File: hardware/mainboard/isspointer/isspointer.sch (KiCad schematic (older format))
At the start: 83 parts, among them J1 USB_B_Micro, J2 Motor 1, J3 Motor 2, Q1 SS8050-G, Q2 SS8050-G, Q3 DMN67D8L, Q4 DMN67D8L, SW1 SW_Push, SW2 SW_Push, U1 AMS1117-3.3, U2 CP2102N-A01-GQFN28, U3 esp32-WROOM-32D, U4 DRV8834_HTSSOP, U5 DRV8834_HTSSOP, U6 LSM303DLHC, U7 EE-SX3350, U8 EE-SX3350

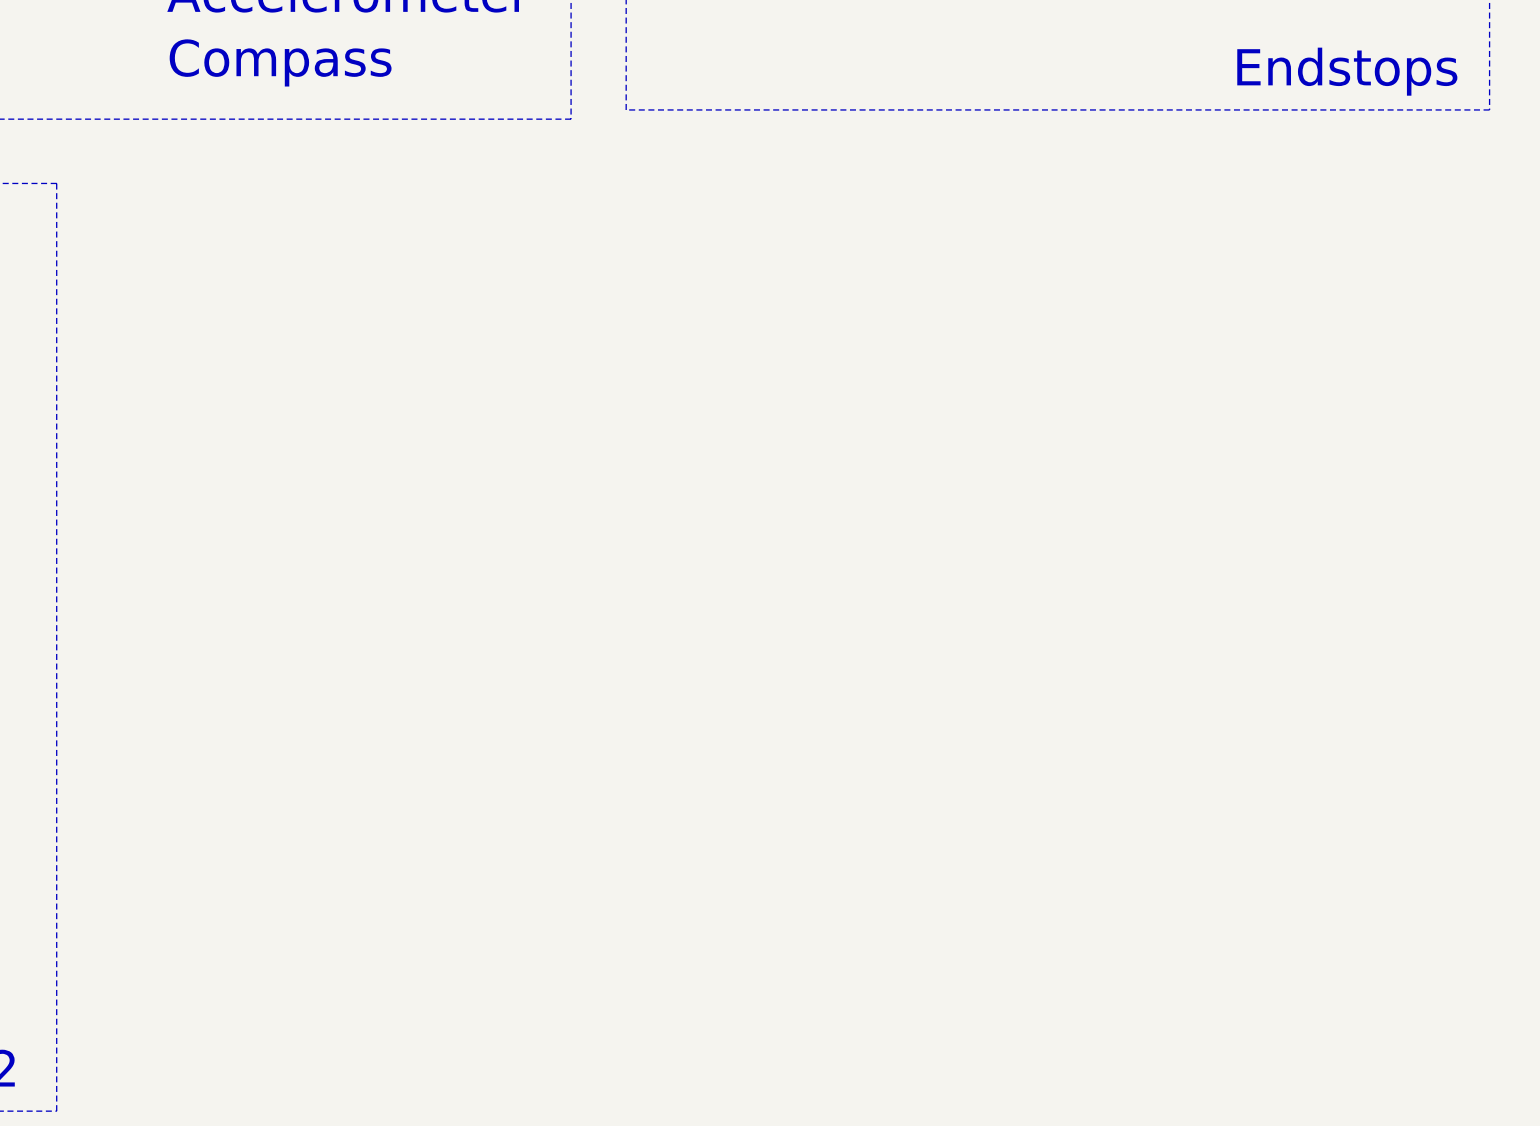
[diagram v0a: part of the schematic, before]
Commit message: display!
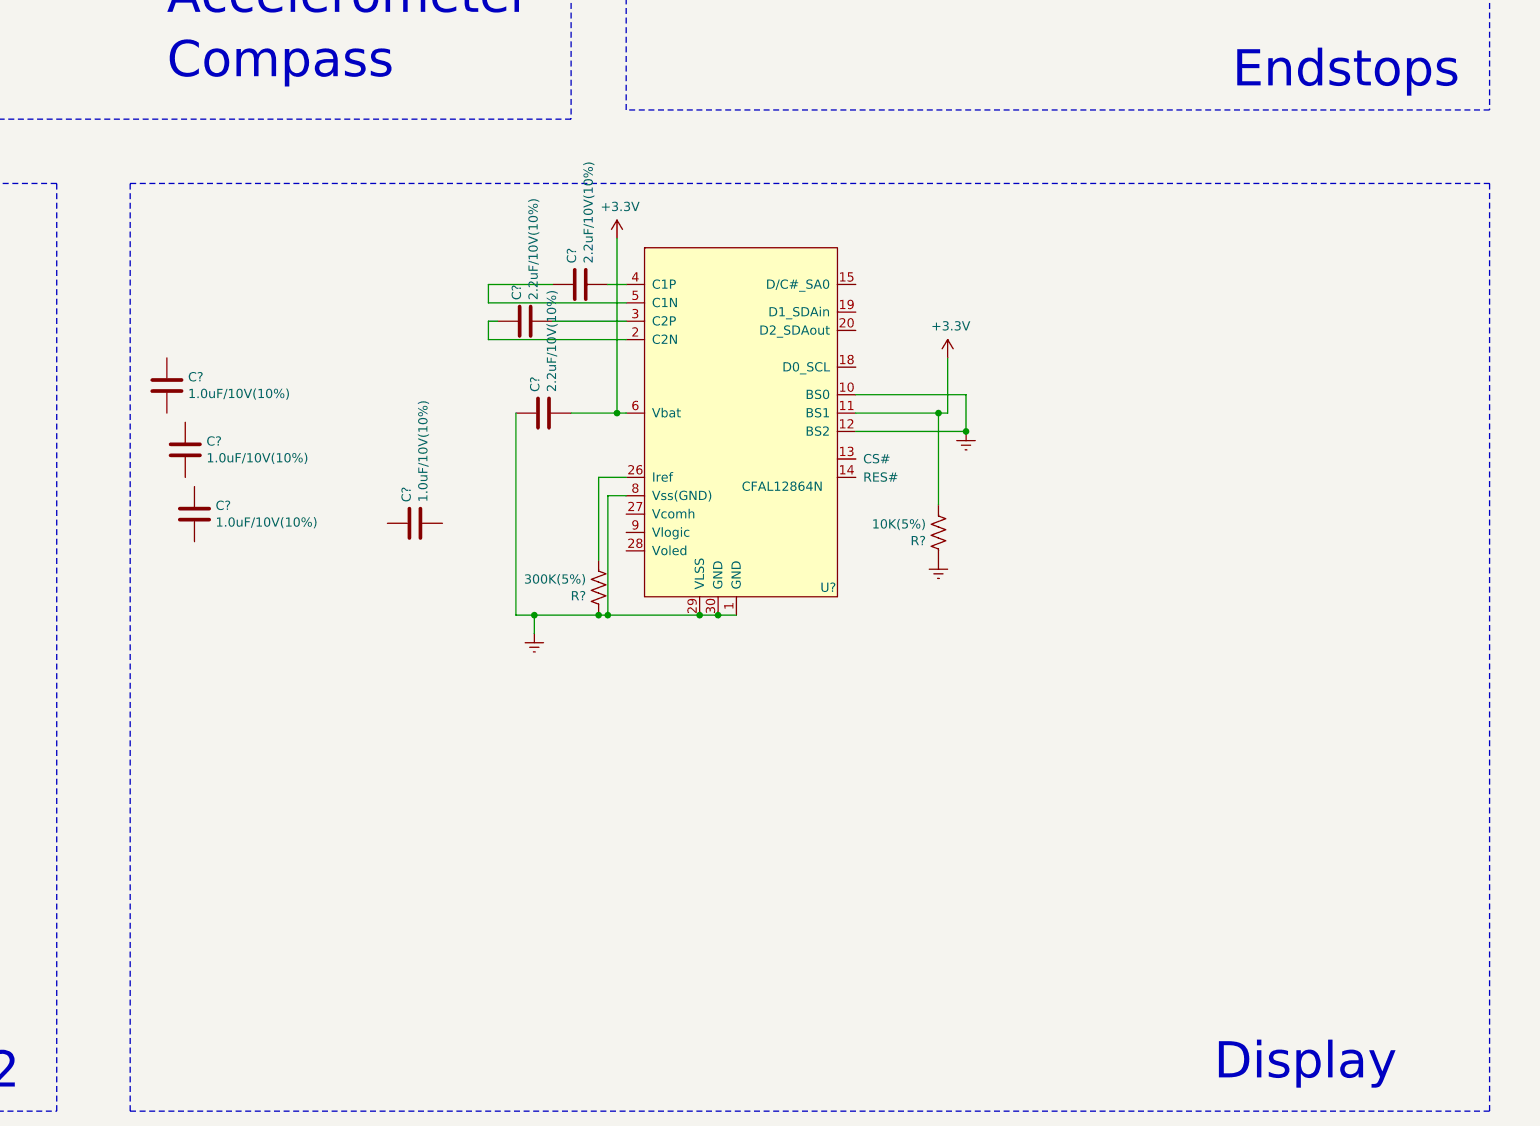
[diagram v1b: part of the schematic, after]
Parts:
- added C? (x4): 1.0uF/10V(10%), Capacitor_SMD:C_0603_1608Metric_Pad1.05x0.95mm_HandSolder, symbol Device:C
- added C? (x3): 2.2uF/10V(10%), Capacitor_SMD:C_0603_1608Metric_Pad1.05x0.95mm_HandSolder, symbol Device:C
- added R?: 300K(5%), Resistor_SMD:R_0603_1608Metric_Pad1.05x0.95mm_HandSolder, symbol Device:R_US
- added R?: 10K(5%), Resistor_SMD:R_0603_1608Metric_Pad1.05x0.95mm_HandSolder, symbol Device:R_US
- added U?: CFAL12864N, symbol isspointer:CFAL12864N
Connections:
- net +3V3: now also C?.2, R?.2, U?.11 (BS1), U?.6 (Vbat)
- net GNDREF: now also C?.1, R?.1, R?.1, U?.1 (GND), U?.10 (BS0), U?.12 (BS2), U?.29 (VLSS), U?.30 (GND), U?.8 (Vss(GND))
- new net: C?.1, U?.2 (C2N)
- new net: C?.2, U?.3 (C2P)
- new net: R?.2, U?.26 (Iref)
- new net: C?.1, U?.5 (C1N)
- new net: C?.2, U?.4 (C1P)
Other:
- note added: "Display"
